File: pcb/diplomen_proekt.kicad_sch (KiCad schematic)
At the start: 27 parts, among them SW1 SW_Push, U1 DA56-11SURKWA, U2 ESP32-S3, U3 HC-SR04, U4 ACTIVE_BUZZER, U5 TP4056, U6 MCP1826S

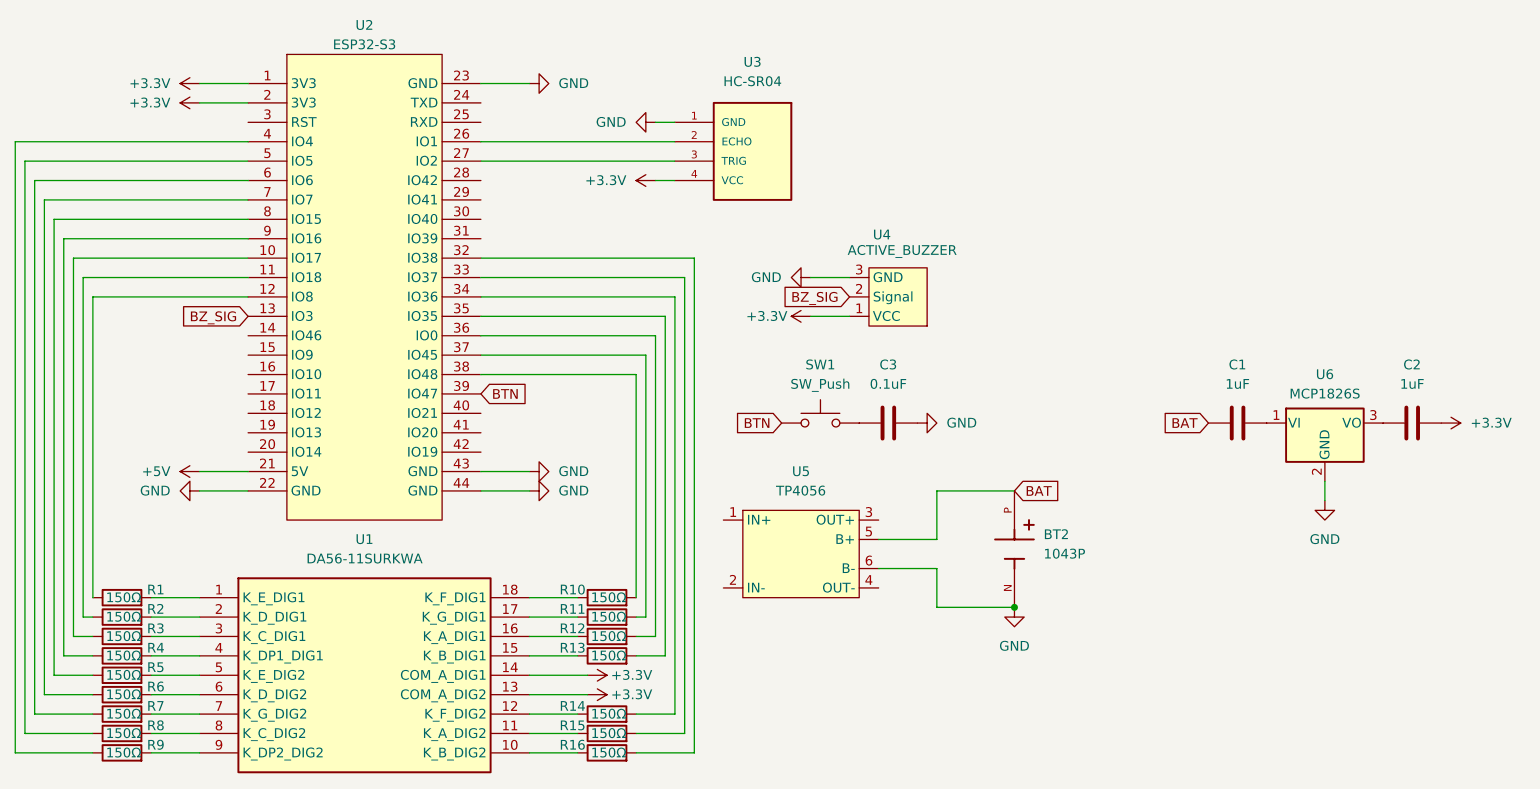
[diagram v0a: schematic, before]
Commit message: Added pcb images
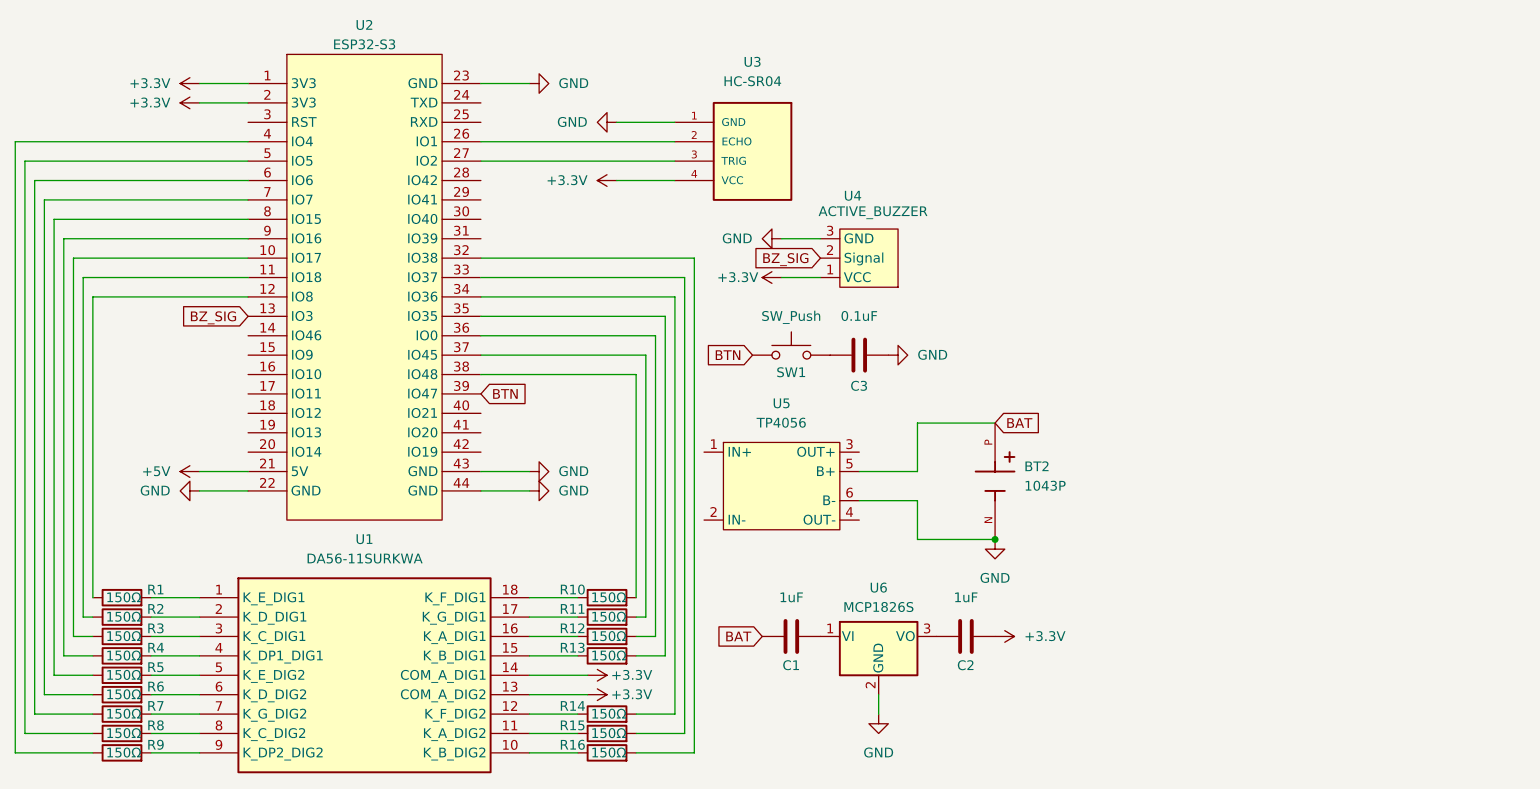
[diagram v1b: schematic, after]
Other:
- moved on the sheet: BT2, C1, C2, C3, SW1, U4, U5, U6
